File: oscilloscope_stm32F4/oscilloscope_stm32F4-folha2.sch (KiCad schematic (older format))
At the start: 35 parts, among them J1 ST-Link, J2 USB_B_Micro, K1 AQY210EH, K2 AQY210EH, P2 CH_1, P5 CH_2, U1 LM1117-3.3, U1 STM32F411CEU6_-_UFQFPN48, U2 MCP6S21-I_SN, U3 MCP6S21-I_SN

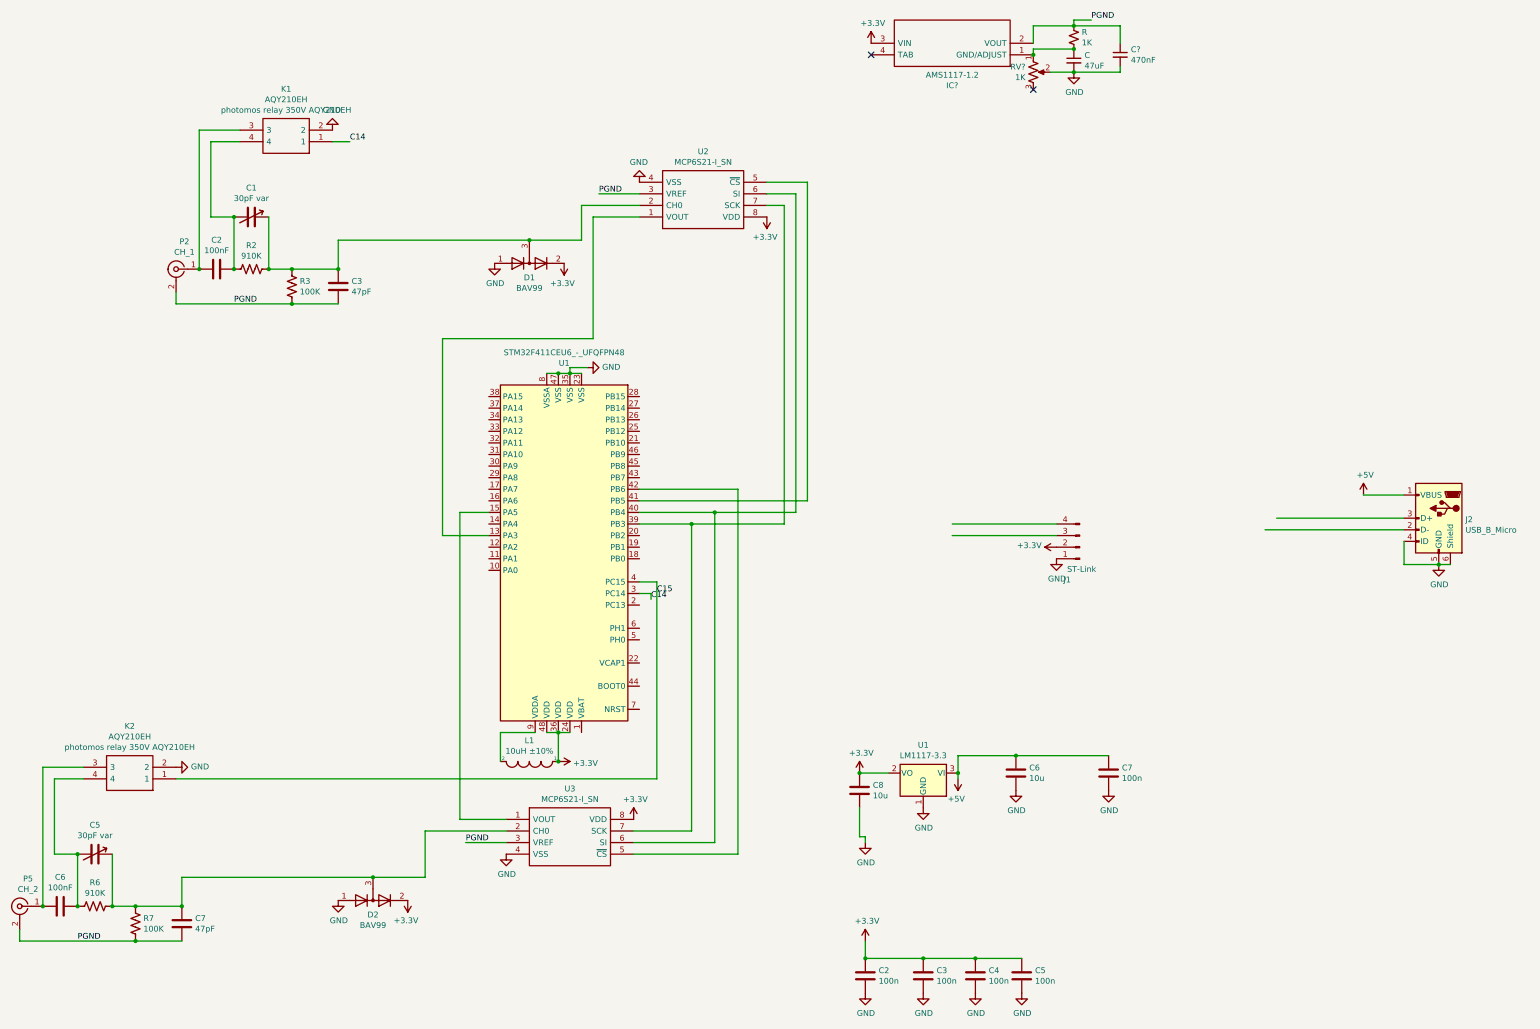
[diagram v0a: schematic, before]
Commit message: atualização
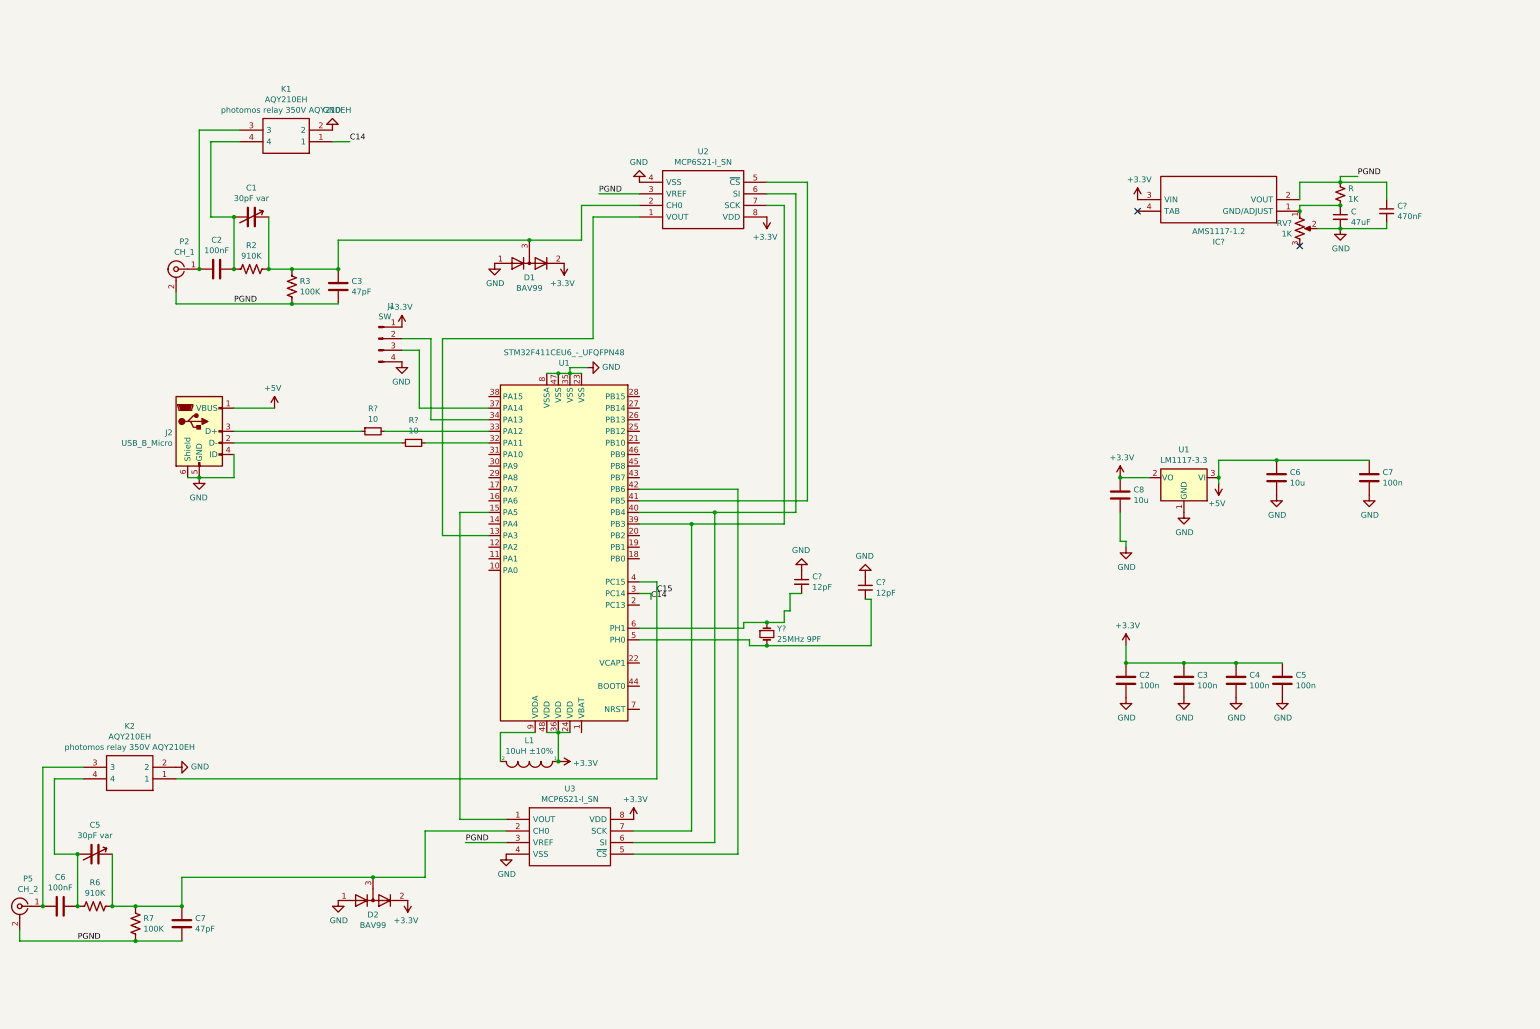
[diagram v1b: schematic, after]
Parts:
- added C? (x2): 12pF, symbol Device:C_Small
- added R? (x2): 10, symbol Device:R_Small
- added Y?: 25MHz 9PF, symbol Device:Crystal_Small
- J1: value ST-Link -> SW
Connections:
- wire segments 109 -> 129
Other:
- moved on the sheet: C, C2, C3, C4, C5, C6, C7, C8, C?, IC?, J1, J2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
